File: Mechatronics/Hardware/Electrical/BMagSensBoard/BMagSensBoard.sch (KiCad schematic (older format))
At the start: 2 parts, among them J1 Conn_01x06_Male, U1 TLE5009

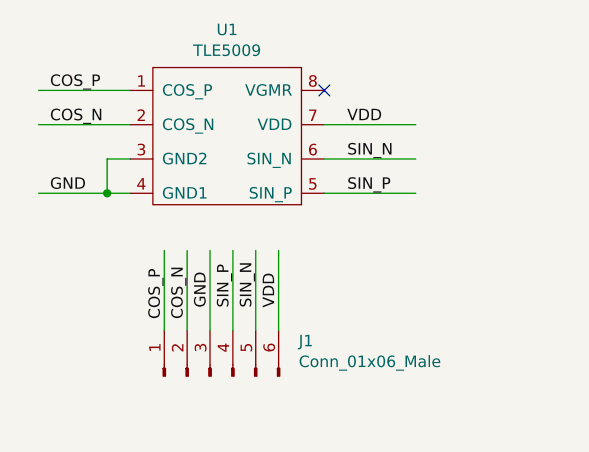
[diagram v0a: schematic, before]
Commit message: Changes
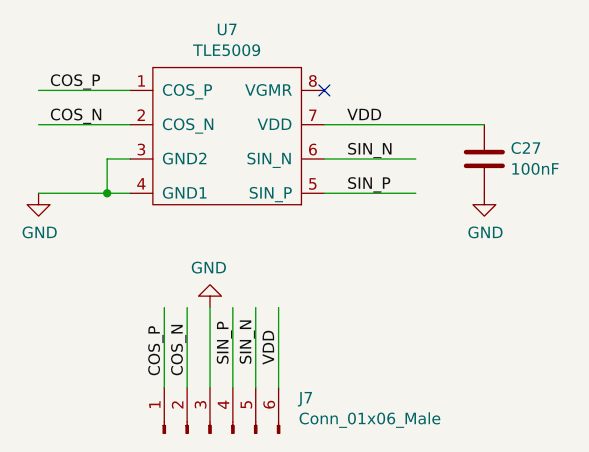
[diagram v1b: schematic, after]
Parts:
- added C27: 100nF, Encoder:C_0603_1608Metric_Pad1.05x0.95mm_HandSolder, symbol Device:C
- renumbered J1 to J7, U1 to U7
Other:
- moved on the sheet: J7
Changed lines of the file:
@@
 $EndDescr
 $Comp
-L Encoder:TLE5009 U1
+L Encoder:TLE5009 U7
 U 1 1 5F0B6CA7
 P 5400 3900
-F 0 "U1" H 5375 4365 50  0000 C CNN
+F 0 "U7" H 5375 4365 50  0000 C CNN
 F 1 "TLE5009" H 5375 4274 50  0000 C CNN
 F 2 "Encoder:SO-8_3.9x4.9mm_P1.27mm" H 5350 3800 50  0001 C CNN
@@
 $EndComp
 $Comp
-L Connector:Conn_01x06_Male J1
+L Connector:Conn_01x06_Male J7
 U 1 1 5F0B758B
-P 5300 4950
-F 0 "J1" V 5454 4562 50  0000 R CNN
-F 1 "Conn_01x06_Male" V 5363 4562 50  0000 R CNN
-F 2 "Encoder:SolderWirePad_1x01_SMD_5x10mm" H 5300 4950 50  0001 C CNN
-F 3 "~" H 5300 4950 50  0001 C CNN
-	1    5300 4950
+P 5300 5200
+F 0 "J7" V 5454 4812 50  0000 R CNN
+F 1 "Conn_01x06_Male" V 5363 4812 50  0000 R CNN
+F 2 "Encoder:SolderWirePad_1x01_SMD_5x10mm" H 5300 5200 50  0001 C CNN
+F 3 "~" H 5300 5200 50  0001 C CNN
+	1    5300 5200
 	0    -1   -1   0
 $EndComp
 Wire Wire Line
-	5100 4750 5100 4400
+	5100 5000 5100 4650
 Wire Wire Line
-	5200 4750 5200 4400
+	5200 5000 5200 4650
 Wire Wire Line
-	5300 4750 5300 4400
+	5300 5000 5300 4650
 Wire Wire Line
-	5400 4750 5400 4400
+	5400 5000 5400 4650
 Wire Wire Line
-	5500 4750 5500 4400
+	5500 5000 5500 4650
 Wire Wire Line
-	5600 4750 5600 4400
+	5600 5000 5600 4650
 Wire Wire Line
 	4950 4150 4850 4150
@@
 Text Label 5900 4150 0    50   ~ 0
 SIN_P
-Text Label 4600 4150 0    50   ~ 0
-GND
 Text Label 4600 3850 0    50   ~ 0
 COS_N
@@
 Wire Wire Line
 	5800 4000 6200 4000
+Text Label 5100 4950 1    50   ~ 0
+COS_P
+Text Label 5200 4950 1    50   ~ 0
+COS_N
+Text Label 5500 4900 1    50   ~ 0
+SIN_N
+Text Label 5400 4900 1    50   ~ 0
+SIN_P
+Text Label 5600 4900 1    50   ~ 0
+VDD
+$Comp
+L Device:C C27
+U 1 1 5F13AC11
+P 6500 4000
+F 0 "C27" H 6615 4046 50  0000 L CNN
+F 1 "100nF" H 6615 3955 50  0000 L CNN
+F 2 "Encoder:C_0603_1608Metric_Pad1.05x0.95mm_HandSolder" H 6538 3850 50  0001 C CNN
+F 3 "~" H 6500 4000 50  0001 C CNN
+	1    6500 4000
+	1    0    0    -1
+$EndComp
+$Comp
+L power:GND #PWR0101
+U 1 1 5F13B1C6
+P 4550 4150
+F 0 "#PWR0101" H 4550 3900 50  0001 C CNN
+F 1 "GND" H 4555 3977 50  0000 C CNN
+F 2 "" H 4550 4150 50  0001 C CNN
+F 3 "" H 4550 4150 50  0001 C CNN
+	1    4550 4150
+	1    0    0    -1
+$EndComp
 Wire Wire Line
-	5800 3850 6200 3850
-Text Label 5100 4700 1    50   ~ 0
-COS_P
-Text Label 5200 4700 1    50   ~ 0
-COS_N
-Text Label 5300 4650 1    50   ~ 0
-GND
-Text Label 5500 4650 1    50   ~ 0
-SIN_N
-Text Label 5400 4650 1    50   ~ 0
-SIN_P
-Text Label 5600 4650 1    50   ~ 0
-VDD
+	5800 3850 6500 3850
+$Comp
+L power:GND #PWR0102
+U 1 1 5F13B564
+P 6500 4150
+F 0 "#PWR0102" H 6500 3900 50  0001 C CNN
+F 1 "GND" H 6505 3977 50  0000 C CNN
+F 2 "" H 6500 4150 50  0001 C CNN
+F 3 "" H 6500 4150 50  0001 C CNN
+	1    6500 4150
+	1    0    0    -1
+$EndComp
+$Comp
+L power:GND #PWR?
+U 1 1 5F13CDDA
+P 5300 4650
+F 0 "#PWR?" H 5300 4400 50  0001 C CNN
+F 1 "GND" H 5305 4477 50  0000 C CNN
+F 2 "" H 5300 4650 50  0001 C CNN
+F 3 "" H 5300 4650 50  0001 C CNN
+	1    5300 4650
+	-1   0    0    1
+$EndComp
 $EndSCHEMATC
